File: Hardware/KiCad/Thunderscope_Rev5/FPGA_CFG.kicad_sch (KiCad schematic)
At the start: 7 parts, among them U18 IC FPGA XC7A50T-2CSG325C

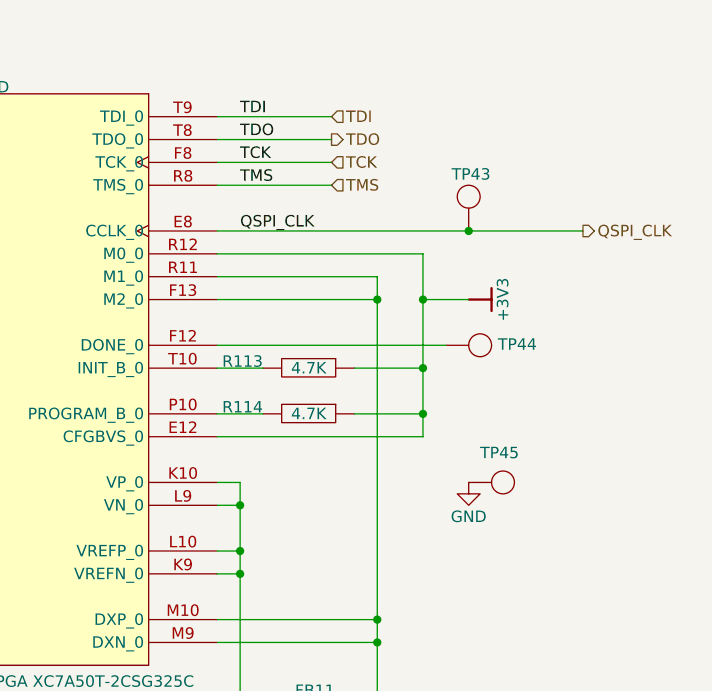
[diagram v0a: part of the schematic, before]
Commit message: Schematic cleanup and RGB status LED
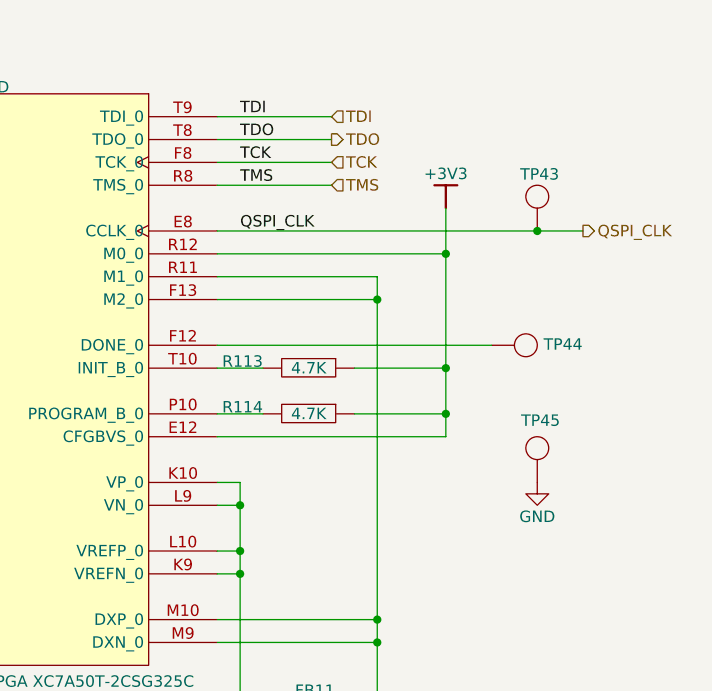
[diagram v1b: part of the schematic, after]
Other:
- moved on the sheet: TP43, TP44, TP45
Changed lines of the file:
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@@
 	)
 	(junction
-		(at 175.26 96.52)
+		(at 177.8 96.52)
 		(diameter 0)
 		(color 0 0 0 0)
@@
 	)
 	(junction
-		(at 180.34 81.28)
+		(at 177.8 101.6)
 		(diameter 0)
 		(color 0 0 0 0)
 	)
 	(junction
-		(at 175.26 101.6)
+		(at 187.96 81.28)
 		(diameter 0)
 		(color 0 0 0 0)
@@
 	)
 	(junction
-		(at 175.26 88.9)
+		(at 177.8 83.82)
 		(diameter 0)
 		(color 0 0 0 0)
@@
 	(wire
 		(pts
-			(xy 152.4 71.12) (xy 165.1 71.12)
+			(xy 187.96 81.28) (xy 193.04 81.28)
 		)
 		(stroke
@@
 	(wire
 		(pts
-			(xy 154.94 119.38) (xy 154.94 116.84)
+			(xy 152.4 71.12) (xy 165.1 71.12)
 		)
 		(stroke
@@
 	(wire
 		(pts
-			(xy 175.26 101.6) (xy 167.64 101.6)
+			(xy 154.94 119.38) (xy 154.94 116.84)
 		)
 		(stroke
@@
 	(wire
 		(pts
-			(xy 170.18 88.9) (xy 152.4 88.9)
+			(xy 177.8 101.6) (xy 167.64 101.6)
 		)
 		(stroke
@@
 	(wire
 		(pts
-			(xy 152.4 119.38) (xy 154.94 119.38)
+			(xy 170.18 88.9) (xy 152.4 88.9)
 		)
 		(stroke
@@
 	(wire
 		(pts
-			(xy 180.34 88.9) (xy 175.26 88.9)
+			(xy 152.4 119.38) (xy 154.94 119.38)
 		)
 		(stroke
@@
 	(wire
 		(pts
-			(xy 175.26 83.82) (xy 152.4 83.82)
+			(xy 177.8 83.82) (xy 152.4 83.82)
 		)
 		(stroke
@@
 	(wire
 		(pts
-			(xy 167.64 96.52) (xy 175.26 96.52)
+			(xy 167.64 96.52) (xy 177.8 96.52)
 		)
 		(stroke
@@
 	(wire
 		(pts
-			(xy 180.34 81.28) (xy 193.04 81.28)
-		)
-		(stroke
-			(width 0)
-			(type default)
-		)
-	)
-	(wire
-		(pts
 			(xy 154.94 116.84) (xy 152.4 116.84)
 		)
@@
 	(wire
 		(pts
-			(xy 175.26 96.52) (xy 175.26 101.6)
+			(xy 177.8 96.52) (xy 177.8 101.6)
 		)
 		(stroke
@@
 	(wire
 		(pts
-			(xy 175.26 88.9) (xy 175.26 83.82)
+			(xy 177.8 78.74) (xy 177.8 83.82)
 		)
 		(stroke
@@
 	(wire
 		(pts
-			(xy 157.48 134.62) (xy 154.94 134.62)
+			(xy 177.8 83.82) (xy 177.8 96.52)
 		)
 		(stroke
@@
 	(wire
 		(pts
-			(xy 175.26 96.52) (xy 175.26 88.9)
+			(xy 157.48 134.62) (xy 154.94 134.62)
 		)
 		(stroke
@@
 	(wire
 		(pts
-			(xy 177.8 93.98) (xy 152.4 93.98)
+			(xy 182.88 93.98) (xy 152.4 93.98)
 		)
 		(stroke
@@
 	(wire
 		(pts
-			(xy 152.4 81.28) (xy 180.34 81.28)
+			(xy 152.4 81.28) (xy 187.96 81.28)
 		)
 		(stroke
@@
 	(wire
 		(pts
-			(xy 175.26 104.14) (xy 175.26 101.6)
+			(xy 177.8 104.14) (xy 177.8 101.6)
 		)
 		(stroke
@@
 	(wire
 		(pts
-			(xy 152.4 104.14) (xy 175.26 104.14)
+			(xy 152.4 104.14) (xy 177.8 104.14)
 		)
 		(stroke
@@
 	(symbol
 		(lib_id "Thunderscope_Rev5:TP PCB 1mm")
-		(at 177.8 93.98 0)
+		(at 182.88 93.98 0)
 		(unit 1)
 		(exclude_from_sim no)
@@
 		(dnp no)
 		(property "Reference" "TP44"
-			(at 183.5827 94.6296 0)
+			(at 188.6627 94.6296 0)
 			(effects
 				(font
@@
 		)
 		(property "Value" "PCB"
-			(at 177.292 92.71 0)
+			(at 182.372 92.71 0)
 			(effects
 				(font
@@
 		)
 		(property "Footprint" "Thunderscope_Rev5:GEN_TP_PCB"
-			(at 177.8 93.98 0)
+			(at 182.88 93.98 0)
 			(effects
 				(font
@@
 		)
 		(property "Datasheet" ""
-			(at 177.8 93.98 0)
+			(at 182.88 93.98 0)
 			(effects
 				(font
@@
 		)
 		(property "Description" ""
-			(at 177.8 93.98 0)
+			(at 182.88 93.98 0)
 			(effects
 				(font
@@
 		)
 		(property "HOUSE PART NUMBER" ""
-			(at 177.292 92.71 0)
+			(at 182.372 92.71 0)
 			(effects
 				(font
@@
 		)
 		(property "MANUFACTURER" ""
-			(at 177.292 92.71 0)
+			(at 182.372 92.71 0)
 			(effects
 				(font
@@
 		)
 		(property "MANUFACTURER PART NUMBER" ""
-			(at 177.292 92.71 0)
+			(at 182.372 92.71 0)
 			(effects
 				(font
@@
 		)
 		(property "ALTIUM_VALUE" ""
-			(at 177.8 93.98 0)
+			(at 182.88 93.98 0)
 			(effects
 				(font
@@
 	(symbol
 		(lib_id "Thunderscope_Rev5:TP PCB 1mm")
-		(at 180.34 81.28 90)
+		(at 187.96 81.28 90)
 		(unit 1)
 		(exclude_from_sim no)
@@
 		(dnp no)
 		(property "Reference" "TP43"
-			(at 182.772 74.2429 90)
+			(at 190.392 74.2429 90)
 			(effects
 				(font
@@
 		)
 		(property "Value" "PCB"
-			(at 175.26 82.55 0)
+			(at 182.88 82.55 0)
 			(effects
 				(font
@@
 		)
 		(property "Footprint" "Thunderscope_Rev5:GEN_TP_PCB"
-			(at 180.34 81.28 0)
+			(at 187.96 81.28 0)
 			(effects
 				(font
@@
 		)
 		(property "Datasheet" ""
-			(at 180.34 81.28 0)
+			(at 187.96 81.28 0)
 			(effects
 				(font
@@
 		)
 		(property "Description" ""
-			(at 180.34 81.28 0)
+			(at 187.96 81.28 0)
 			(effects
 				(font
@@
 		)
 		(property "HOUSE PART NUMBER" ""
-			(at 175.26 82.55 0)
+			(at 182.88 82.55 0)
 			(effects
 				(font
@@
 		)
 		(property "MANUFACTURER" ""
-			(at 175.26 82.55 0)
+			(at 182.88 82.55 0)
 			(effects
 				(font
@@
 		)
 		(property "MANUFACTURER PART NUMBER" ""
-			(at 175.26 82.55 0)
+			(at 182.88 82.55 0)
 			(effects
 				(font
@@
 		)
 		(property "ALTIUM_VALUE" ""
-			(at 180.34 81.28 0)
+			(at 187.96 81.28 0)
 			(effects
 				(font
@@
 	(symbol
 		(lib_id "Thunderscope_Rev5:+3V3_BAR")
-		(at 180.34 88.9 90)
+		(at 177.8 78.74 180)
 		(unit 1)
 		(exclude_from_sim no)
@@
 		(dnp no)
 		(property "Reference" "#PWR0279"
-			(at 180.34 88.9 0)
+			(at 177.8 78.74 0)
 			(effects
 				(font
@@
 		)
 		(property "Value" "+3V3"
-			(at 184.15 88.9 0)
+			(at 177.8 74.93 0)
 			(effects
 				(font
@@
 		)
 		(property "Footprint" ""
-			(at 180.34 88.9 0)
+			(at 177.8 78.74 0)
 			(effects
 				(font
@@
 		)
 		(property "Datasheet" ""
-			(at 180.34 88.9 0)
+			(at 177.8 78.74 0)
 			(effects
 				(font
@@
 		)
 		(property "Description" "Power symbol creates a global label with name '+3V3'"
-			(at 180.34 88.9 0)
+			(at 177.8 78.74 0)
 			(effects
 				(font
@@
 	(symbol
 		(lib_id "Thunderscope_Rev5:TP PCB 1mm")
-		(at 180.34 109.22 0)
+		(at 187.96 109.22 90)
 		(unit 1)
 		(exclude_from_sim no)
@@
 		(dnp no)
 		(property "Reference" "TP45"
-			(at 181.61 106.68 0)
+			(at 190.5 101.6 90)
 			(effects
 				(font
@@
 		)
 		(property "Value" "PCB"
-			(at 179.07 104.14 0)
+			(at 182.88 110.49 0)
 			(effects
 				(font
@@
 		)
 		(property "Footprint" "Thunderscope_Rev5:GEN_TP_PCB"
-			(at 180.34 109.22 0)
+			(at 187.96 109.22 0)
 			(effects
 				(font
@@
 		)
 		(property "Datasheet" ""
-			(at 180.34 109.22 0)
+			(at 187.96 109.22 0)
 			(effects
 				(font
@@
 		)
 		(property "Description" ""
-			(at 180.34 109.22 0)
+			(at 187.96 109.22 0)
 			(effects
 				(font
@@
 		)
 		(property "HOUSE PART NUMBER" ""
-			(at 177.8 101.6 0)
+			(at 180.34 111.76 0)
 			(effects
 				(font
@@
 		)
 		(property "MANUFACTURER" ""
-			(at 177.8 101.6 0)
+			(at 180.34 111.76 0)
 			(effects
 				(font
@@
 		)
 		(property "MANUFACTURER PART NUMBER" ""
-			(at 177.8 101.6 0)
+			(at 180.34 111.76 0)
 			(effects
 				(font
@@
 		)
 		(property "ALTIUM_VALUE" ""
-			(at 180.34 109.22 0)
+			(at 187.96 109.22 0)
 			(effects
 				(font
@@
 	(symbol
 		(lib_id "Thunderscope_Rev5:GND")
-		(at 180.34 109.22 0)
+		(at 187.96 109.22 0)
 		(unit 1)
 		(exclude_from_sim no)
@@
 		(dnp no)
 		(property "Reference" "#PWR0503"
-			(at 180.34 115.57 0)
+			(at 187.96 115.57 0)
 			(effects
 				(font
@@
 		)
 		(property "Value" "GND"
-			(at 180.34 113.03 0)
+			(at 187.96 113.03 0)
 			(effects
 				(font
@@
 		)
 		(property "Footprint" ""
-			(at 180.34 109.22 0)
+			(at 187.96 109.22 0)
 			(effects
 				(font
@@
 		)
 		(property "Datasheet" ""
-			(at 180.34 109.22 0)
+			(at 187.96 109.22 0)
 			(effects
 				(font
@@
 		)
 		(property "Description" "Power symbol creates a global label with name \"GND\" , ground"
-			(at 180.34 109.22 0)
+			(at 187.96 109.22 0)
 			(effects
 				(font
